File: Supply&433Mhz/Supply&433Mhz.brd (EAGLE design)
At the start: 65 x 56.5 mm, 19 parts, among them IC1 3.3V, K1 61004021821, P1 DF11-06-2DS, Q1 BS170

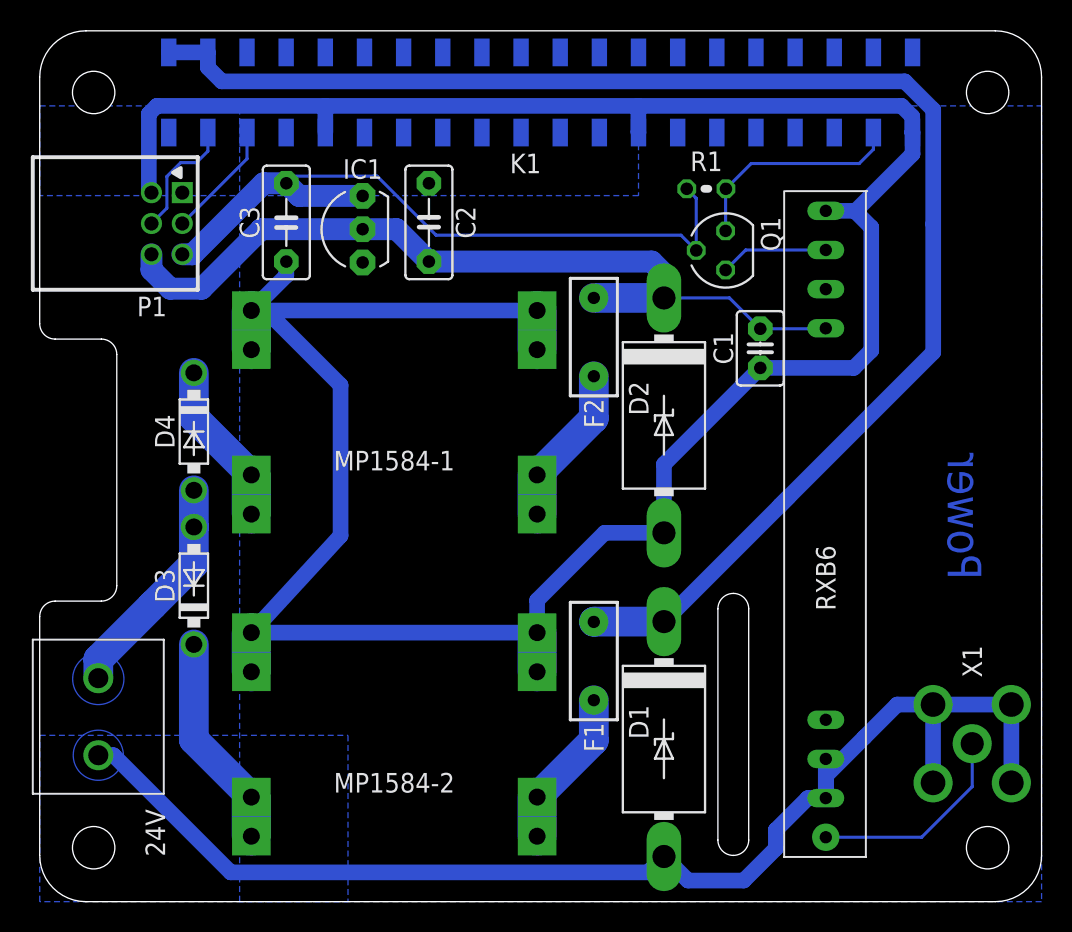
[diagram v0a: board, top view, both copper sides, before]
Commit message: Minor.
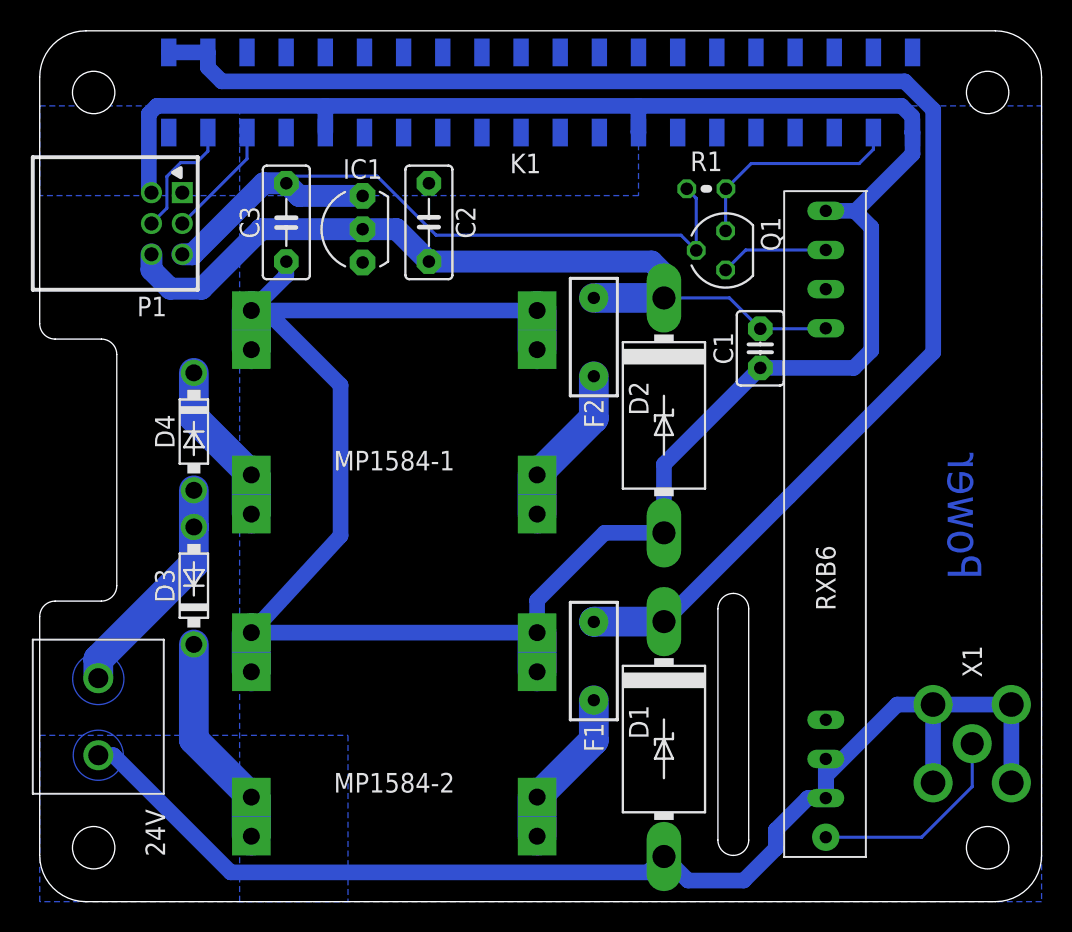
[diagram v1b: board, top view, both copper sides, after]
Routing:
- net N$5: track 97.5 -> 96.7 mm
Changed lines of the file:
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@@
 <wire x1="19.52" y1="23.745" x2="13.729" y2="17.454" width="1.016" layer="16"/>
 <wire x1="51" y1="6.72" x2="51" y2="8.16" width="1.016" layer="16"/>
-<wire x1="51" y1="8.16" x2="53.51" y2="10.67" width="1.016" layer="16"/>
-<wire x1="53.51" y1="10.67" x2="55.63" y2="12.79" width="1.016" layer="16"/>
+<wire x1="51" y1="8.16" x2="55.63" y2="12.79" width="1.016" layer="16"/>
 <wire x1="55.63" y1="12.79" x2="57.96" y2="12.79" width="1.016" layer="16"/>
 <wire x1="56.63" y1="49.9" x2="56.63" y2="48.51" width="1.016" layer="16"/>
@@
 <wire x1="10" y1="26.69" x2="10" y2="24.31" width="1.9304" layer="16"/>
 <wire x1="10" y1="24.31" x2="10" y2="21.92" width="1.9304" layer="16"/>
-<wire x1="10" y1="21.92" x2="7.32" y2="19.24" width="1.9304" layer="16"/>
-<wire x1="7.32" y1="19.24" x2="3.8" y2="15.72" width="1.9304" layer="16"/>
+<wire x1="10" y1="21.92" x2="3.8" y2="15.72" width="1.9304" layer="16"/>
 <wire x1="3.8" y1="15.72" x2="3.8" y2="14.5" width="1.9304" layer="16"/>
 </signal>
@@
 <wire x1="48.035" y1="25.705" x2="48.62" y2="26.29" width="1.016" layer="16"/>
 <wire x1="56.13" y1="53.22" x2="57.97" y2="51.38" width="1.016" layer="16"/>
-<wire x1="57.97" y1="51.38" x2="57.97" y2="43.97" width="1.016" layer="16"/>
-<wire x1="57.97" y1="43.97" x2="57.97" y2="35.64" width="1.016" layer="16"/>
-<wire x1="57.97" y1="35.64" x2="48.035" y2="25.705" width="1.016" layer="16"/>
+<wire x1="57.97" y1="51.38" x2="57.97" y2="35.64" width="1.016" layer="16"/>
+<wire x1="57.97" y1="35.64" x2="48.62" y2="26.29" width="1.016" layer="16"/>
 <wire x1="35.95" y1="18.15" x2="35.98" y2="18.17" width="1.9304" layer="16"/>
 <wire x1="35.98" y1="18.17" x2="40.5" y2="18.17" width="1.9304" layer="16"/>
@@
 <wire x1="16.02" y1="46.61" x2="16" y2="46.61" width="0.2032" layer="16"/>
 <wire x1="16.02" y1="46.61" x2="16.48" y2="47.07" width="0.2032" layer="16"/>
-<wire x1="16.48" y1="47.07" x2="21.63" y2="47.07" width="0.2032" layer="16"/>
-<wire x1="21.63" y1="47.07" x2="21.89" y2="47.07" width="0.2032" layer="16"/>
+<wire x1="16.48" y1="47.07" x2="21.89" y2="47.07" width="0.2032" layer="16"/>
 <wire x1="21.89" y1="47.07" x2="25.72" y2="43.24" width="0.2032" layer="16"/>
 <wire x1="25.72" y1="43.24" x2="41.605" y2="43.24" width="0.2032" layer="16"/>
